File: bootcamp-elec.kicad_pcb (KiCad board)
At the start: 2 copper layers, 23.1 x 32 mm, 17 parts, among them J3 FTDI, SW1 SW_Push, U1 ATmega328P-A, Y1 16MHz

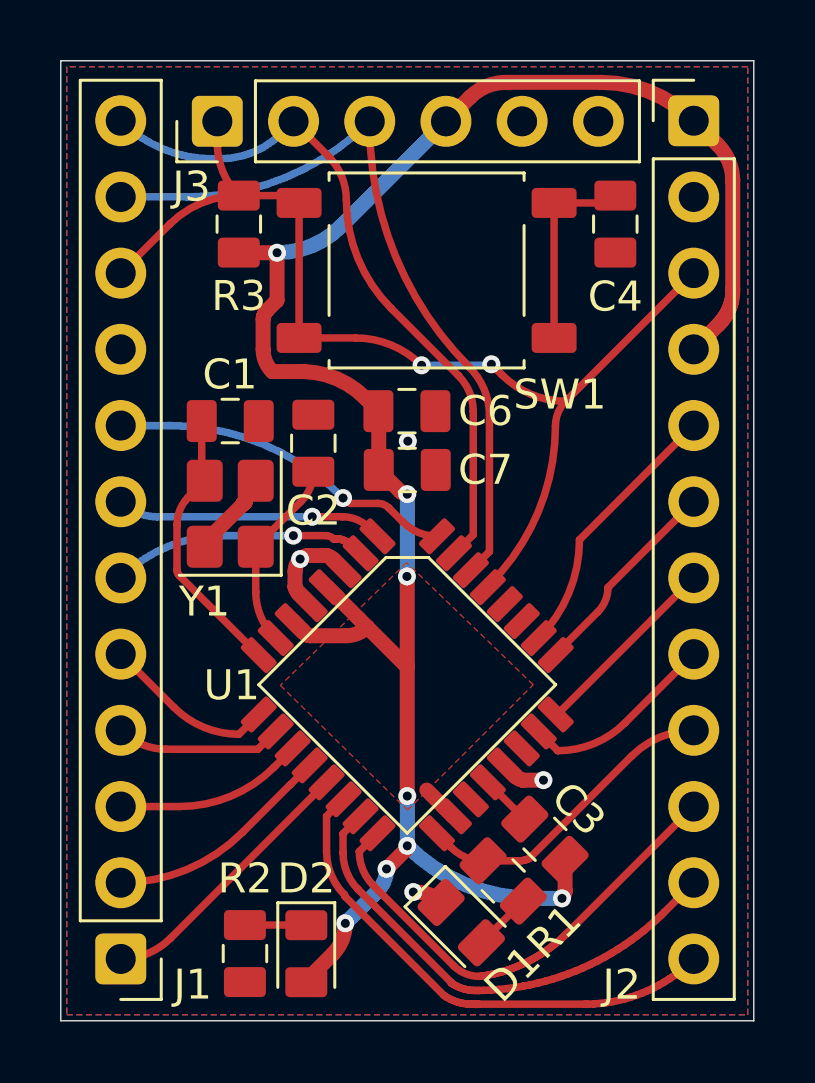
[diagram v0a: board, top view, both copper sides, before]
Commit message: pcb design v3
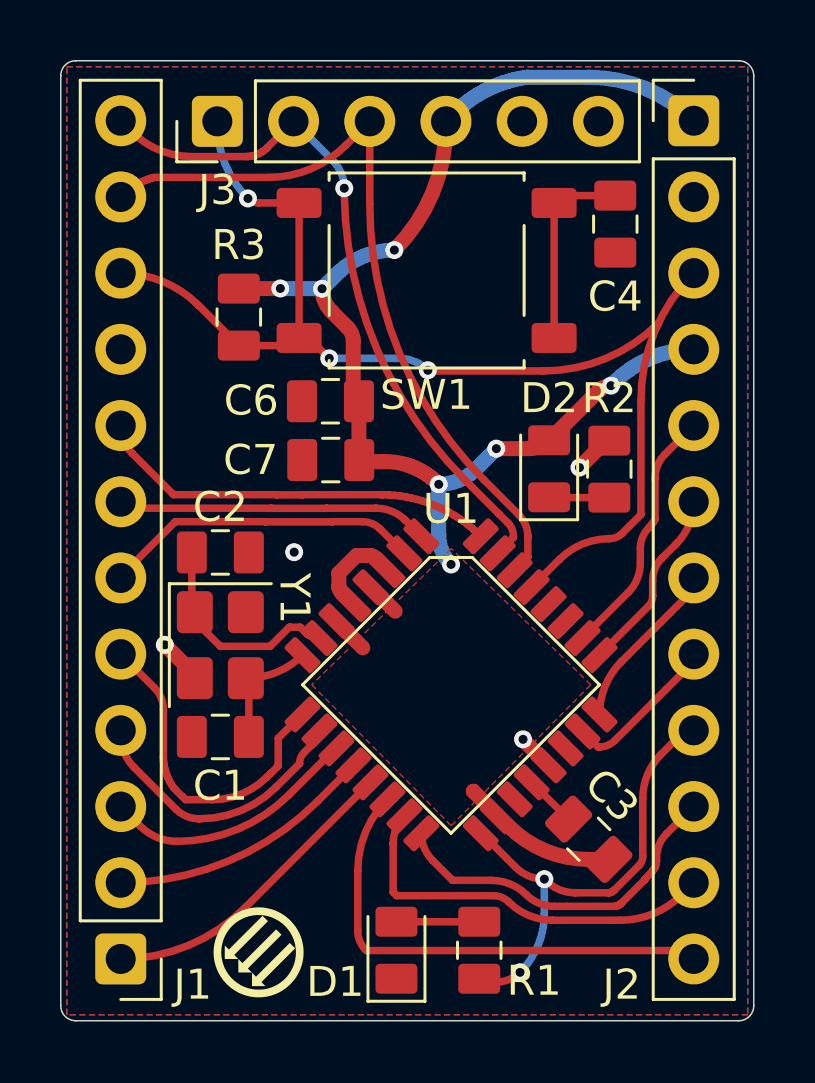
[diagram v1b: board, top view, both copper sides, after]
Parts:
- added G***: LOGO, bootcamp-elec:arrows-silkscreen, F.Cu at (94.6, 74.7)
- moved R2 20.2 mm to (106.3, 58.6), turned to 90 degrees
- moved D2 18.1 mm to (104.3, 58.6), turned to 90 degrees
- moved C1 10.5 mm to (93.3, 67.5), turned to 180 degrees
- moved C2 4.78 mm to (93.3, 61.4), turned to 0 degrees
- moved Y1 4.39 mm to (93.3, 64.5), turned to -90 degrees
- moved R3 3.10 mm to (93.9, 53.5), turned to 90 degrees
- moved C6 2.57 mm to (97.0, 56.4), turned to 0 degrees
- moved C7 2.57 mm to (97.0, 58.3), turned to 180 degrees
- moved R1 2.44 mm to (102.0, 74.7), turned to -90 degrees
- moved D1 2.35 mm to (99.2, 74.7), turned to 90 degrees
- moved U1 1.46 mm to (101.0, 65.8)
- moved C3 1.46 mm to (105.6, 71.0)
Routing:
- net RAW: track 70.1 -> 50.5 mm, vias 8 -> 7
- net SCK: track 10.5 -> 15.9 mm, vias 0 -> 2
- net DTR: track 36.4 -> 41.6 mm, vias 2 -> 3
- net D5: track 6.08 -> 11.1 mm
- net Net-(U1-XTAL2/PB7): track 9.26 -> 4.37 mm
- net MISO: track 16.1 -> 12.0 mm
- net D6: track 5.57 -> 9.41 mm
- net MOSI: track 16.5 -> 13.5 mm
- net D7: track 6.32 -> 8.62 mm
- net D2: track 11.8 -> 13.8 mm, vias 1 -> 0
- net D4: track 9.00 -> 10.5 mm, vias 1 -> 0
- net A1: track 6.48 -> 4.97 mm
- net GND: track 8.81 -> 7.39 mm
- net D9: track 9.19 -> 10.5 mm
- net D8: track 7.64 -> 8.93 mm
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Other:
- outline, holes or cut-outs redrawn
